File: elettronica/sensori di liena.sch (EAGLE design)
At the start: 23 parts, among them J2 2X6, J3 455-1750-1-ND, T1 BP103

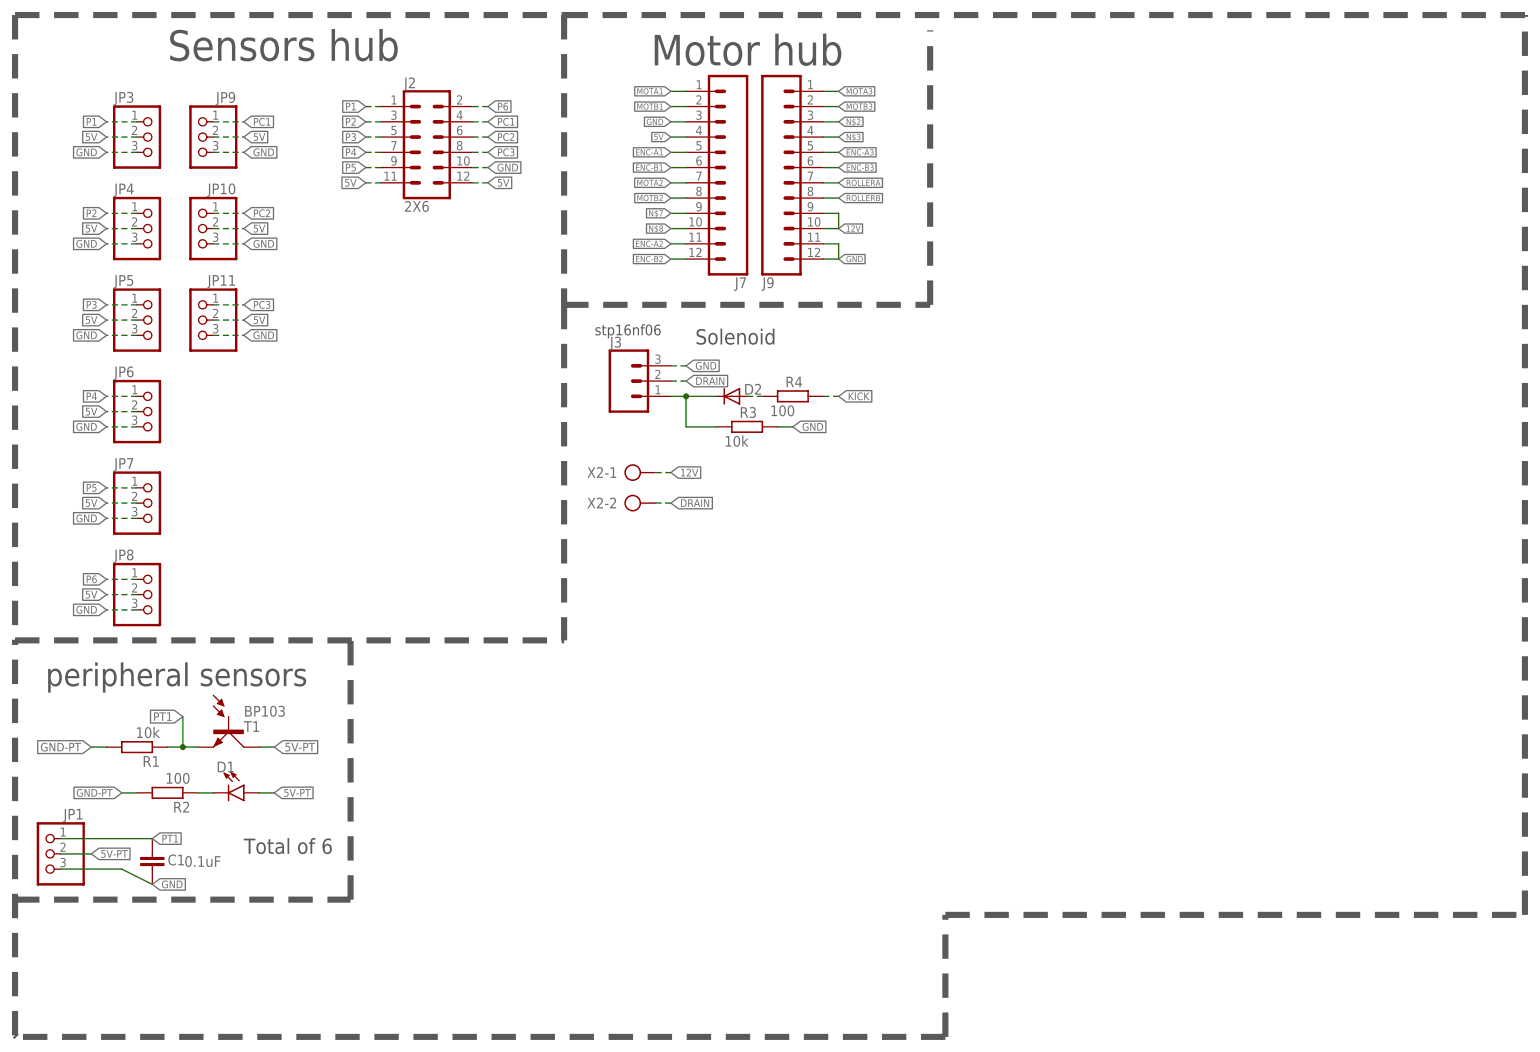
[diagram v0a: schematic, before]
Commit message: sensori di linea done
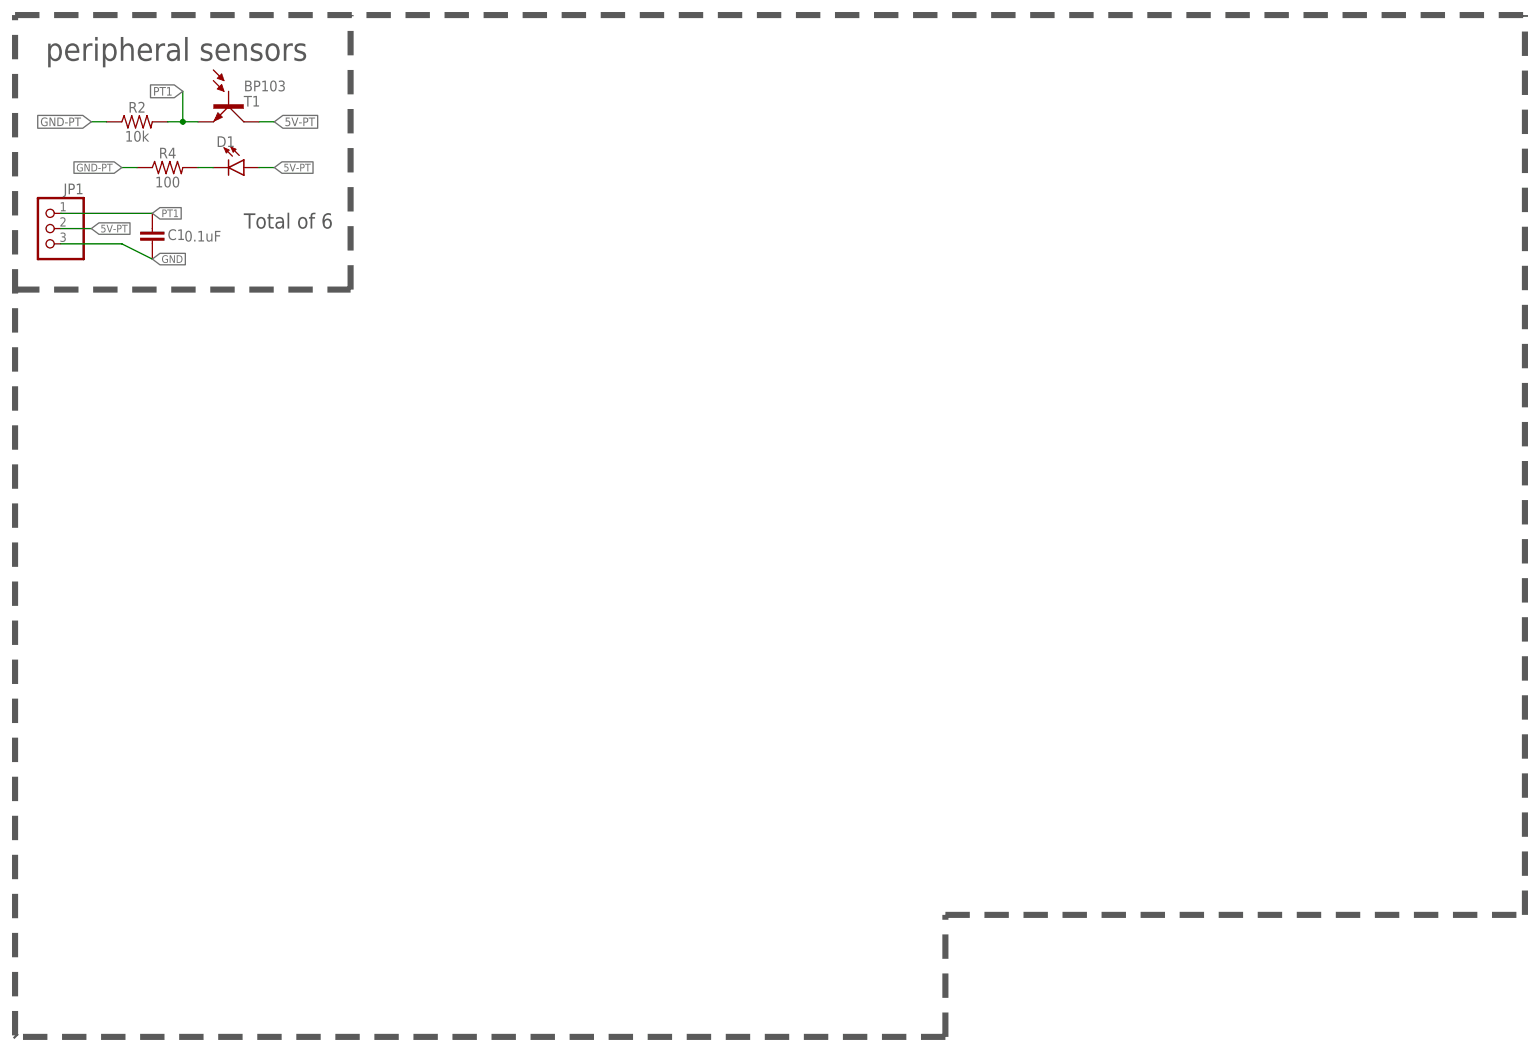
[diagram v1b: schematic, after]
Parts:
- removed D2: 1N4148, diode:1N4148DO35-7
- removed J2: 2X6, SparkFun-Connectors:CONN_06X2PTH_FEMALE
- removed J3: 455-1750-1-ND, SparkFun-Connectors:CONN_03
- removed J7, J9: (no value), SparkFun-Connectors:CONN_12
- removed JP10, JP11, JP3, JP4, JP5, JP6, JP7, JP8, JP9: (no value), pinhead:PINHD-1X3
- removed R1: 10k, eagle-ltspice:R0204/7
- removed R3: 10k, eagle-ltspice:RR1206
- removed X2: (no value), con-ptr500:AK500/2-H
- R2: value 100 -> 10k; device eagle-ltspice:R0204/7 -> SparkFun-Resistors:10KOHM-0603-1/10W-1%
- R4: device eagle-ltspice:RR1206 -> SparkFun-Resistors:10KOHM-0603-1/10W-1%
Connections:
- removed net 12V: J9.10, J9.9, X2-1.KL
- removed net 5V: J2.11, J2.12, J7.4, JP10.2, JP11.2, JP3.2, JP4.2, JP5.2, JP6.2, JP7.2, JP8.2, JP9.2
- removed net DRAIN: J3.2, X2-2.KL
- removed net ENC-A1: J7.5
- removed net ENC-A2: J7.11
- removed net ENC-A3: J9.5
- removed net ENC-B1: J7.6
- removed net ENC-B2: J7.12
- removed net ENC-B3: J9.6
- removed net KICK: R4.2
- removed net MOTA1: J7.1
- removed net MOTA2: J7.7
- removed net MOTA3: J9.1
- removed net MOTB1: J7.2
- removed net MOTB2: J7.8
- removed net MOTB3: J9.2
- removed net N$3: J9.4
- removed net N$4: D2.C, J3.1, R3.1
- removed net N$5: D2.A, R4.1
- removed net N$7: J7.9
- removed net N$8: J7.10
- removed net P1: J2.1, JP3.1
- removed net P2: J2.3, JP4.1
- removed net P3: J2.5, JP5.1
- removed net P4: J2.7, JP6.1
- removed net P5: J2.9, JP7.1
- removed net P6: J2.2, JP8.1
- removed net PC1: J2.4, JP9.1
- removed net PC2: J2.6, JP10.1
- removed net PC3: J2.8, JP11.1
- removed net ROLLERA: J9.7
- removed net ROLLERB: J9.8
- net GND: no longer J2.10, J3.3, J7.3, J9.11, J9.12, JP10.3, JP11.3, JP3.3, JP4.3, JP5.3, JP6.3, JP7.3, JP8.3, JP9.3, R3.2
- net GND-PT: now also R2.1, R4.1; no longer R1.2, R2.2
- net N$2: now also R4.2; no longer J9.3, R2.1
- net PT1: now also R2.2; no longer R1.1
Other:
- note removed: "Motor hub"
- note removed: "Sensors hub"
- note removed: "Solenoid"
- note removed: "stp16nf06"
- moved on the sheet: C1, D1, JP1, T1
